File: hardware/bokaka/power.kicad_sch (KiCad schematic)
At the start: 5 parts, among them U1 AP2112K-3.3

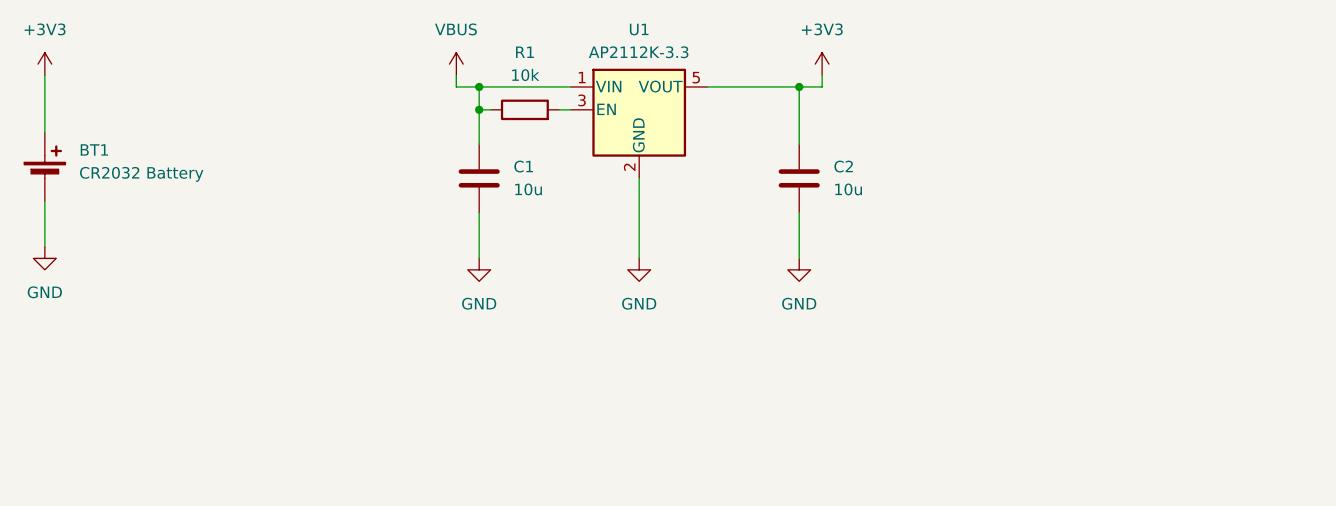
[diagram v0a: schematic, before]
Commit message: Adding rest of design and pdf
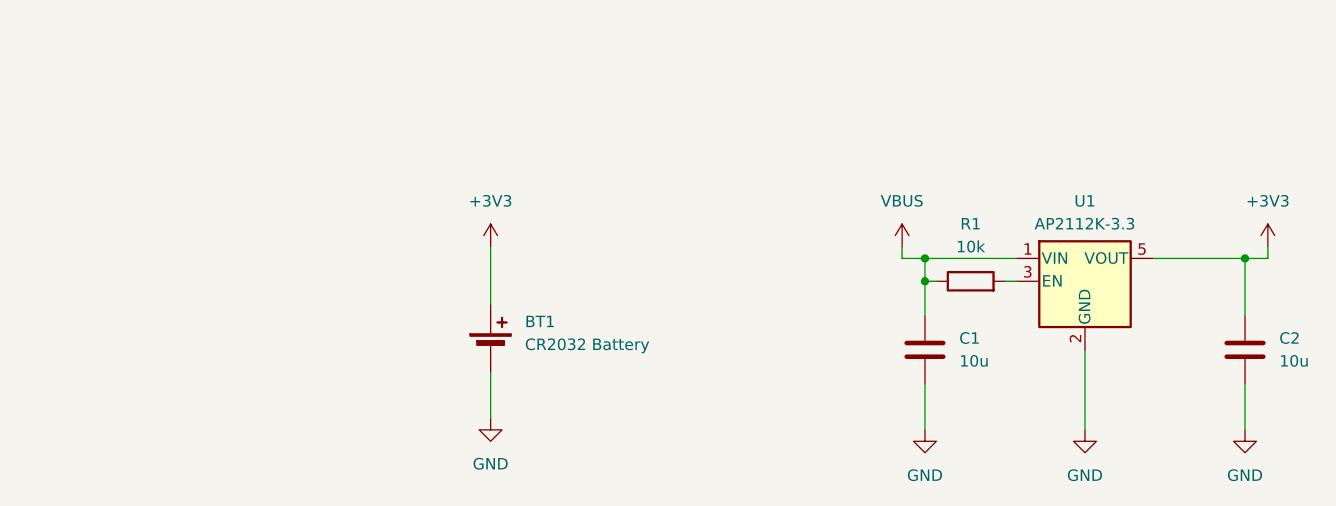
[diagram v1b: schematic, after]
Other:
- moved on the sheet: BT1, C1, C2, R1, U1
